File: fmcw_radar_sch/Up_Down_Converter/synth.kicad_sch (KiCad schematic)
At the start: 6 parts, among them J7 Conn_01x01_Pin, U9 ADF4372BCCZ

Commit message: layout
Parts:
- C1, C2, C3, C4: footprint (none) -> Capacitor_SMD:C_0603_1608Metric_Pad1.08x0.95mm_HandSolder
- J7: footprint (none) -> Connector_PinHeader_2.54mm:PinHeader_1x01_P2.54mm_Vertical
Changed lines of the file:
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@@
 			)
 		)
-		(property "Footprint" ""
+		(property "Footprint" "Capacitor_SMD:C_0603_1608Metric_Pad1.08x0.95mm_HandSolder"
 			(at 203.5048 54.61 0)
 			(effects
@@
 			)
 		)
-		(property "Footprint" ""
+		(property "Footprint" "Capacitor_SMD:C_0603_1608Metric_Pad1.08x0.95mm_HandSolder"
 			(at 72.0852 67.31 0)
 			(effects
@@
 			)
 		)
-		(property "Footprint" ""
+		(property "Footprint" "Capacitor_SMD:C_0603_1608Metric_Pad1.08x0.95mm_HandSolder"
 			(at 175.26 60.6552 0)
 			(effects
@@
 			)
 		)
-		(property "Footprint" ""
+		(property "Footprint" "Capacitor_SMD:C_0603_1608Metric_Pad1.08x0.95mm_HandSolder"
 			(at 186.3852 54.61 0)
 			(effects
@@
 			)
 		)
-		(property "Footprint" ""
+		(property "Footprint" "Connector_PinHeader_2.54mm:PinHeader_1x01_P2.54mm_Vertical"
 			(at 214.63 62.23 0)
 			(effects

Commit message: changes
changes
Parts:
- U9: footprint CC-48-4_ADI -> RF_extra:CC-48-4_ADI
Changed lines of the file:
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@@
 			)
 		)
-		(property "Footprint" "CC-48-4_ADI"
+		(property "Footprint" "RF_extra:CC-48-4_ADI"
 			(at 102.87 46.99 0)
 			(effects

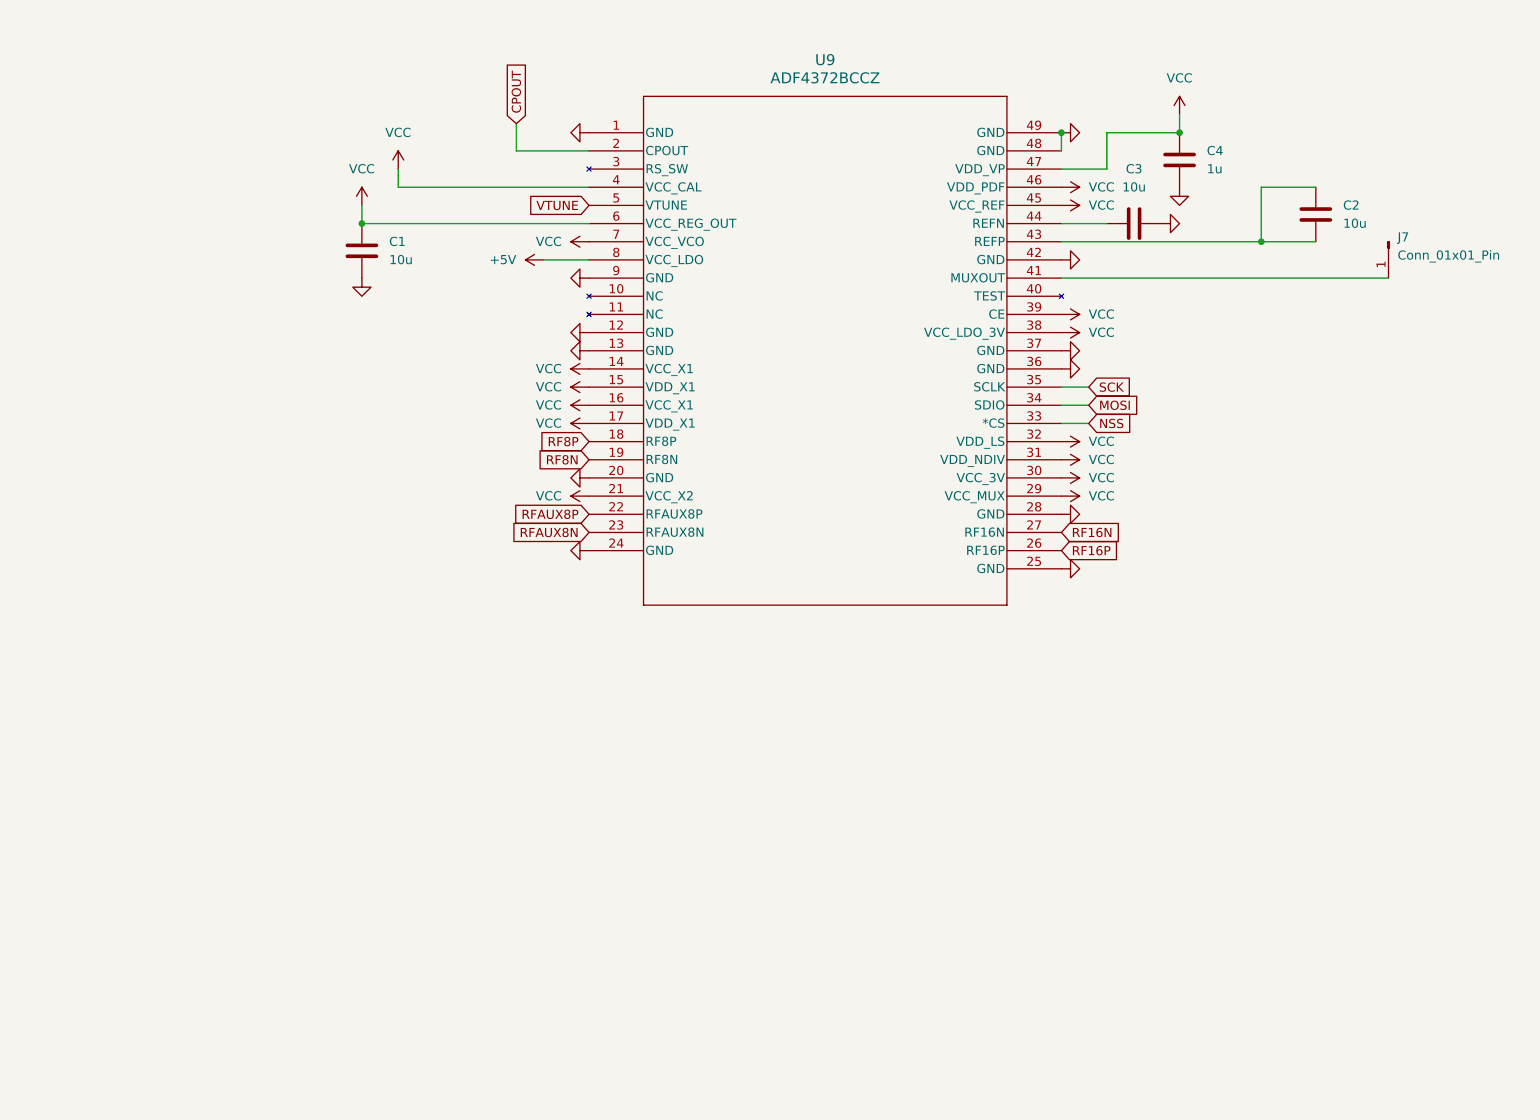
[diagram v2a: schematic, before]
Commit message: a lot of updates
usb power delivery + finishing touches
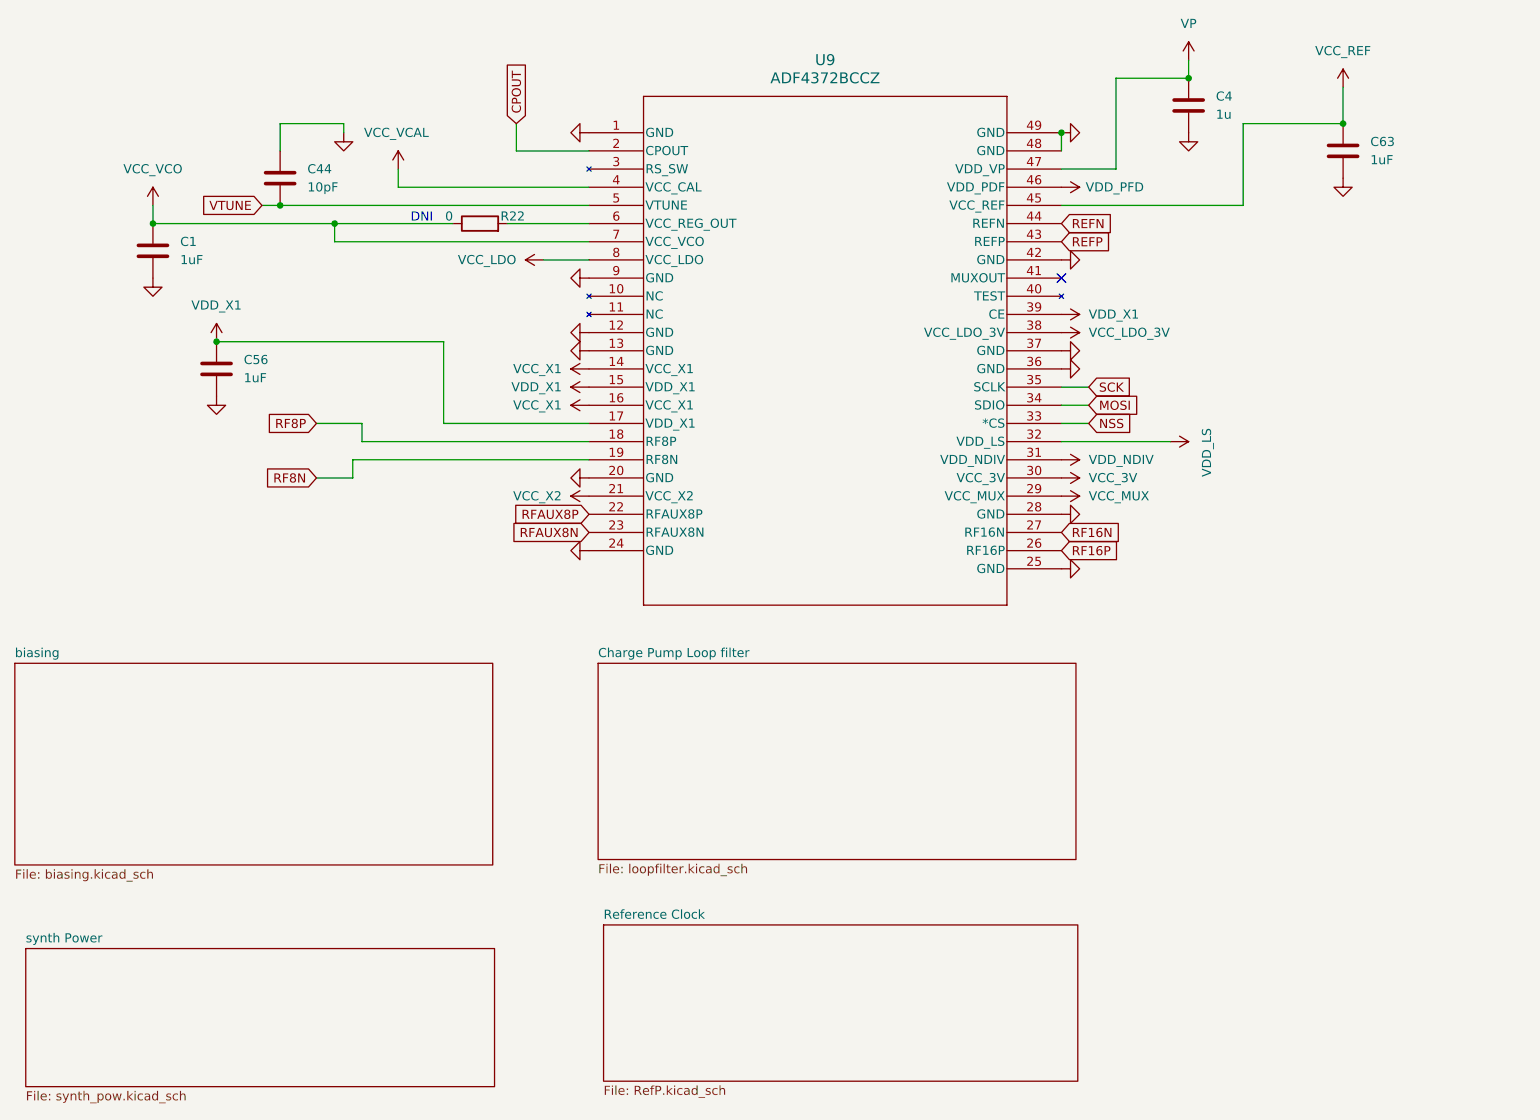
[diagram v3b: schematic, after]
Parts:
- removed C2, C3: 10u, Capacitor_SMD:C_0603_1608Metric_Pad1.08x0.95mm_HandSolder, symbol Device:C
- removed J7: Conn_01x01_Pin, Connector_PinHeader_2.54mm:PinHeader_1x01_P2.54mm_Vertical, symbol Connector:Conn_01x01_Pin
- added C44: 10pF, symbol Device:C
- added C56, C63: 1uF, Capacitor_SMD:C_0603_1608Metric_Pad1.08x0.95mm_HandSolder, symbol Device:C
- added R22: 0, symbol Device:R
- C1: value 10u -> 1uF
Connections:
- net GND: now also C44.1, C56.2, C63.2
- net VTUNE: now also C44.2
- net REFP: now reaches U9.43 (REFP)
- net REFN: now reaches U9.44 (REFN)
- net +5V renamed VCC_LDO
- removed net VCC: C1.1, C4.1, U9.14 (VCC_X1), U9.15 (VDD_X1), U9.16 (VCC_X1), U9.17 (VDD_X1), U9.21 (VCC_X2), U9.29 (VCC_MUX), U9.30 (VCC_3V), U9.31 (VDD_NDIV), U9.32 (VDD_LS), U9.38 (VCC_LDO_3V), U9.39 (CE), U9.4 (VCC_CAL), U9.45 (VCC_REF), U9.46 (VDD_PDF), U9.47 (VDD_VP), U9.6 (VCC_REG_OUT), U9.7 (VCC_VCO)
- new net: R22.2, U9.6 (VCC_REG_OUT)
- new net VCC_3V: U9.30 (VCC_3V)
- new net VCC_LDO_3V: U9.38 (VCC_LDO_3V)
- new net VCC_MUX: U9.29 (VCC_MUX)
- new net VCC_REF: C63.1, U9.45 (VCC_REF)
- new net VCC_VCAL: U9.4 (VCC_CAL)
- new net VCC_VCO: C1.1, R22.1, U9.7 (VCC_VCO)
- new net VCC_X1: U9.14 (VCC_X1), U9.16 (VCC_X1)
- new net VCC_X2: U9.21 (VCC_X2)
- new net VDD_LS: U9.32 (VDD_LS)
- new net VDD_NDIV: U9.31 (VDD_NDIV)
- new net VDD_PFD: U9.46 (VDD_PDF)
- new net VDD_X1: C56.1, U9.15 (VDD_X1), U9.17 (VDD_X1), U9.39 (CE)
- new net VP: C4.1, U9.47 (VDD_VP)
- no-connect marks 0 -> 1
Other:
- added sheet Charge Pump Loop filter (loopfilter.kicad_sch)
- added sheet Reference Clock (RefP.kicad_sch)
- added sheet biasing (biasing.kicad_sch)
- added sheet synth Power (synth_pow.kicad_sch)
- note added: "DNI"
- moved on the sheet: C1, C4

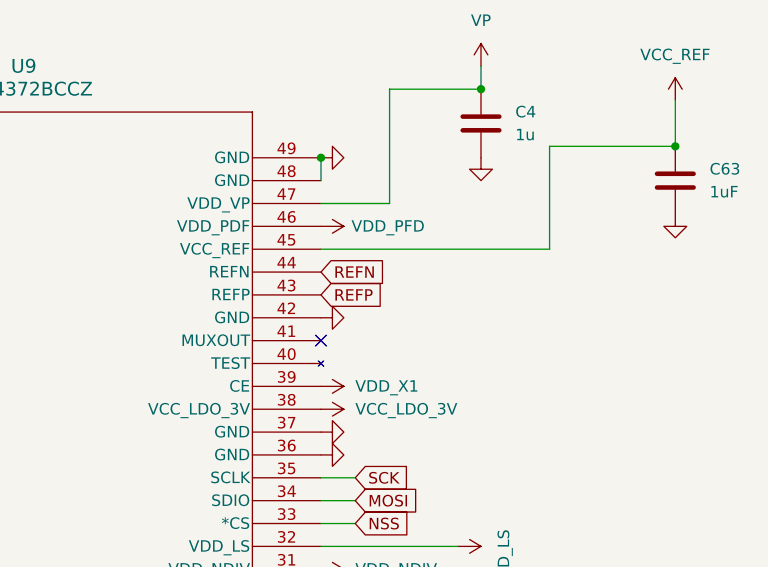
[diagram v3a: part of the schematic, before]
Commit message: Silkscreen finishing
Silkscreen finishting
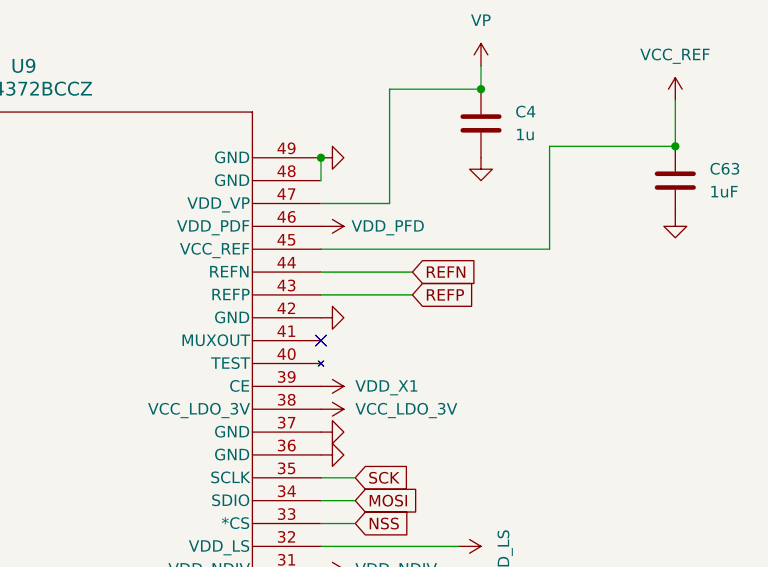
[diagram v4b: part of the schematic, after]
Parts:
- C44: footprint (none) -> Capacitor_SMD:C_0603_1608Metric_Pad1.08x0.95mm_HandSolder
- R22: footprint (none) -> Resistor_SMD:R_0603_1608Metric_Pad0.98x0.95mm_HandSolder
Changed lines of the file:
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@@
 	(wire
 		(pts
+			(xy 179.07 62.23) (xy 168.91 62.23)
+		)
+		(stroke
+			(width 0)
+			(type default)
+		)
+	)
+	(wire
+		(pts
 			(xy 64.77 87.63) (xy 71.12 87.63)
 		)
@@
 		)
 	)
+	(wire
+		(pts
+			(xy 179.07 59.69) (xy 168.91 59.69)
+		)
+		(stroke
+			(width 0)
+			(type default)
+		)
+	)
 	(global_label "RF16P"
 		(shape input)
@@
 		)
 	)
+	(global_label "REFN"
+		(shape input)
+		(at 179.07 59.69 0)
+		(fields_autoplaced yes)
+		(effects
+			(font
+				(size 1.27 1.27)
+			)
+			(justify left)
+		)
+		(property "Intersheetrefs" "${INTERSHEET_REFS}"
+			(at 186.8933 59.69 0)
+			(effects
+				(font
+					(size 1.27 1.27)
+				)
+				(justify left)
+				(hide yes)
+			)
+		)
+	)
 	(global_label "RFAUX8N"
 		(shape input)
@@
 	(global_label "REFP"
 		(shape input)
-		(at 168.91 62.23 0)
+		(at 179.07 62.23 0)
 		(effects
 			(font
@@
 		)
 		(property "Intersheetrefs" "${INTERSHEET_REFS}"
-			(at 168.91 62.23 0)
-			(effects
-				(font
-					(size 1.27 1.27)
-				)
-				(hide yes)
-			)
-		)
-	)
-	(global_label "REFN"
-		(shape input)
-		(at 168.91 59.69 0)
-		(effects
-			(font
-				(size 1.27 1.27)
-			)
-			(justify left)
-		)
-		(property "Intersheetrefs" "${INTERSHEET_REFS}"
-			(at 168.91 59.69 0)
+			(at 179.07 62.23 0)
 			(effects
 				(font
@@
 			)
 		)
-		(property "Footprint" ""
+		(property "Footprint" "Resistor_SMD:R_0603_1608Metric_Pad0.98x0.95mm_HandSolder"
 			(at 87.63 61.468 90)
 			(effects
@@
 			)
 		)
-		(property "Footprint" ""
+		(property "Footprint" "Capacitor_SMD:C_0603_1608Metric_Pad1.08x0.95mm_HandSolder"
 			(at 60.6552 57.15 0)
 			(effects
